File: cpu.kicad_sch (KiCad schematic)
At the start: 17 parts, among them J1 FTSH-105-01-L-DV-K, U2 CC1312R1F3RGZR, Y2 OW7EL89CANUXK7YLC-48M

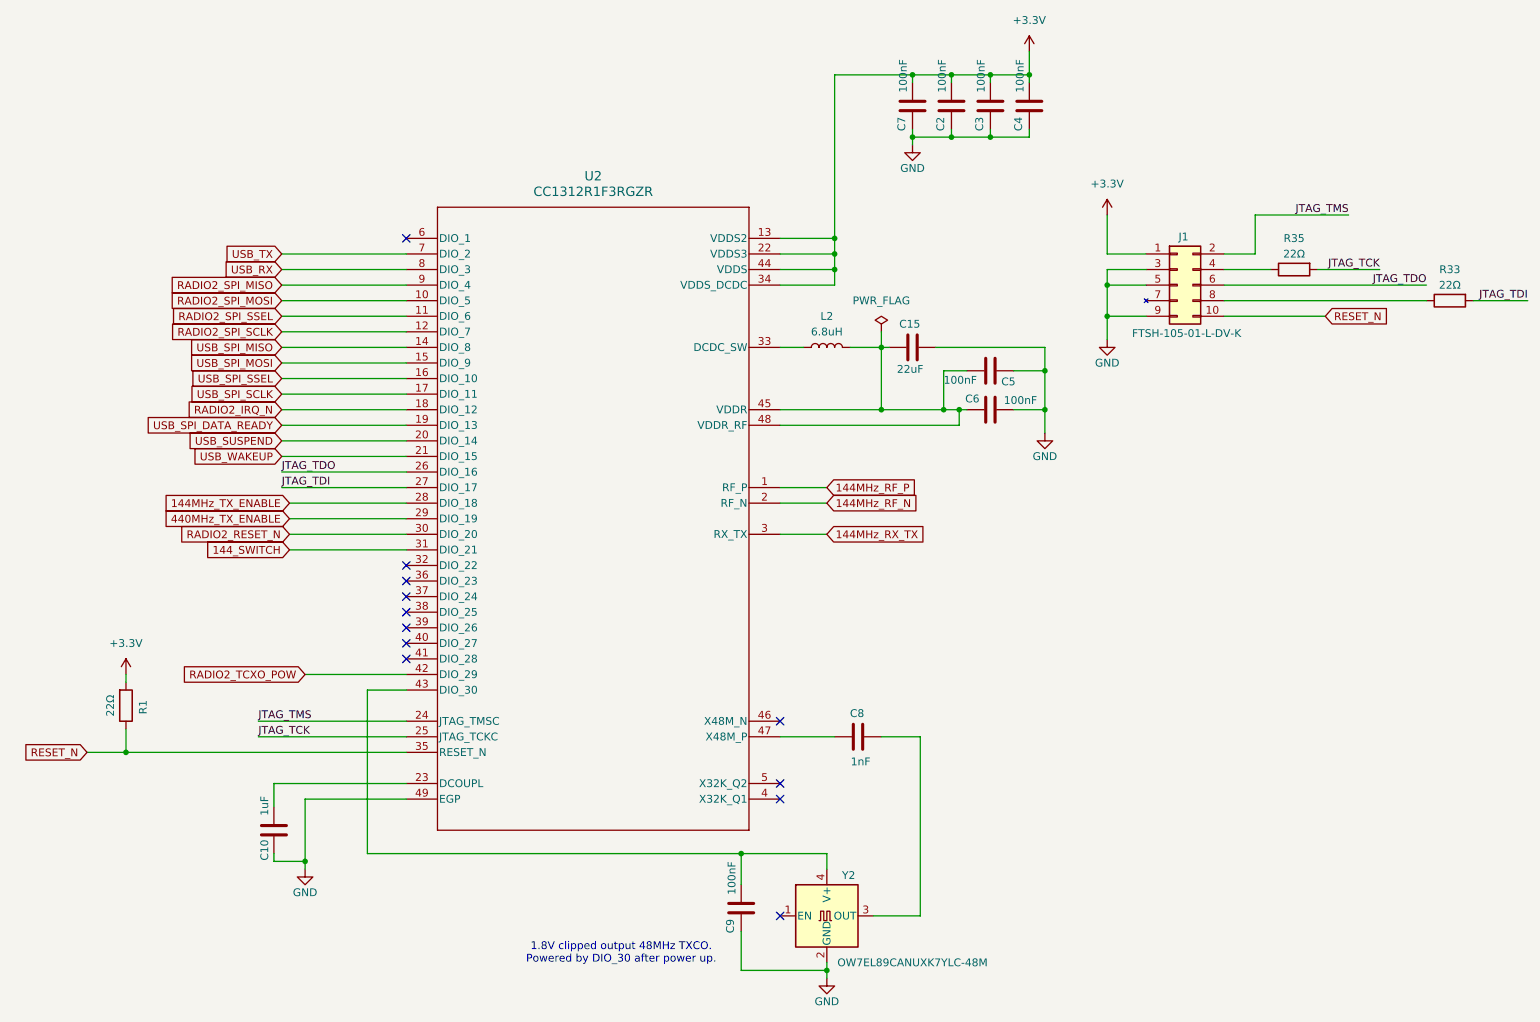
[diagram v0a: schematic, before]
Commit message: Finish layout
Signed-off-by: Corey Minyard <corey@minyard.net>
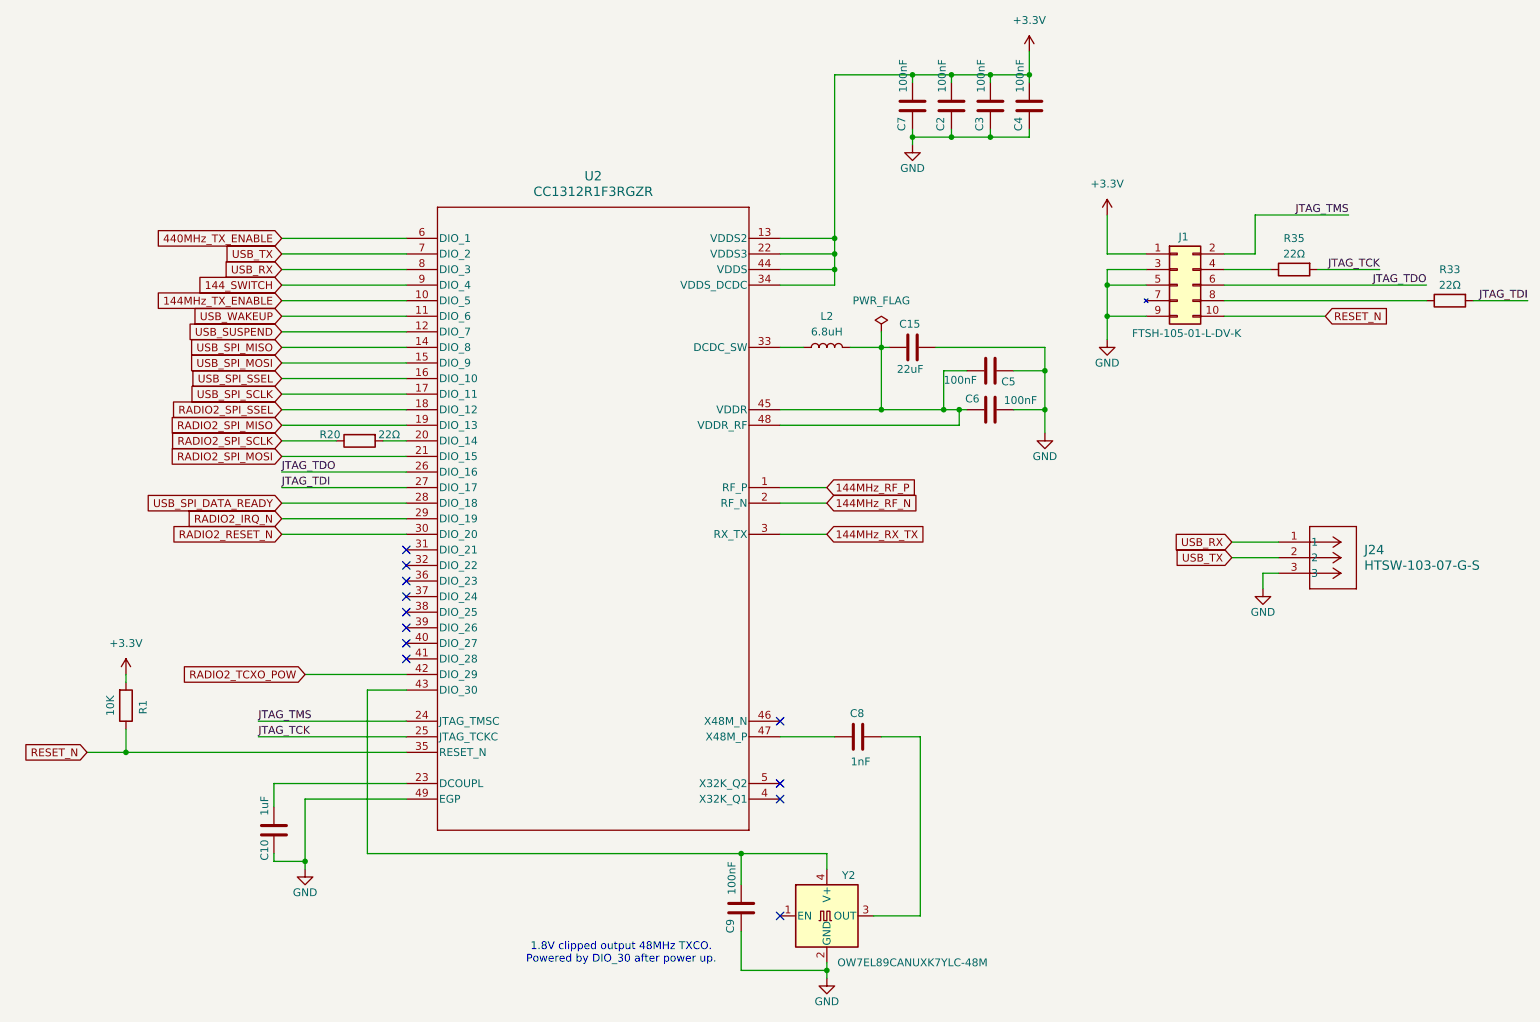
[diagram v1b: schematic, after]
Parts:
- added J24: HTSW-103-07-G-S, CON3_1X3_TU_TSW, symbol Local Connectors:HTSW-103-07-G-S
- added R20: 22Ω, Resistor_SMD:R_0402_1005Metric, symbol Device:R
- R1: value 22Ω -> 10K
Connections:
- net 144MHz_TX_ENABLE: now also U2.10 (DIO_5); no longer U2.28 (DIO_18)
- net 144_SWITCH: now also U2.9 (DIO_4); no longer U2.31 (DIO_21)
- net 440MHz_TX_ENABLE: now also U2.6 (DIO_1); no longer U2.29 (DIO_19)
- net GND: now also J24.3
- net RADIO2_IRQ_N: now also U2.29 (DIO_19); no longer U2.18 (DIO_12)
- net RADIO2_SPI_MISO: now also U2.19 (DIO_13); no longer U2.9 (DIO_4)
- net RADIO2_SPI_MOSI: now also U2.21 (DIO_15); no longer U2.10 (DIO_5)
- net RADIO2_SPI_SCLK: now also R20.1; no longer U2.12 (DIO_7)
- net RADIO2_SPI_SSEL: now also U2.18 (DIO_12); no longer U2.11 (DIO_6)
- net USB_RX: now also J24.1
- net USB_SPI_DATA_READY: now also U2.28 (DIO_18); no longer U2.19 (DIO_13)
- net USB_SUSPEND: now also U2.12 (DIO_7); no longer U2.20 (DIO_14)
- net USB_TX: now also J24.2
- net USB_WAKEUP: now also U2.11 (DIO_6); no longer U2.21 (DIO_15)
- new net: R20.2, U2.20 (DIO_14)
